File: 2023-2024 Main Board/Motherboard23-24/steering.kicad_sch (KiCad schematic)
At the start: 5 parts, among them J1 Conn_01x06_Pin, J18 Conn_01x02_Pin, J19 Conn_01x03_Pin, J7 Conn_01x03_Pin, U1 ARDUINO_PRO_MINI

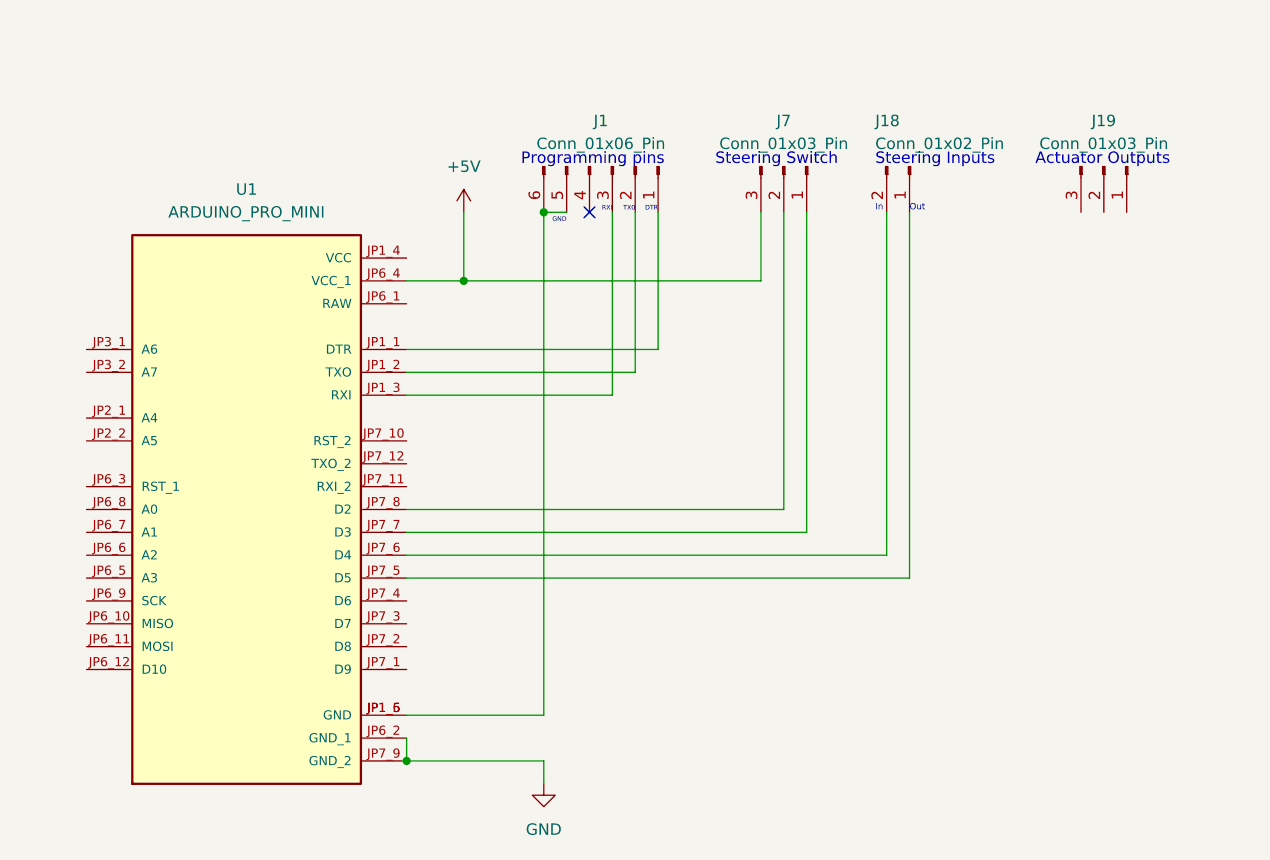
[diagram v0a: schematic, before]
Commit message: Added BOM
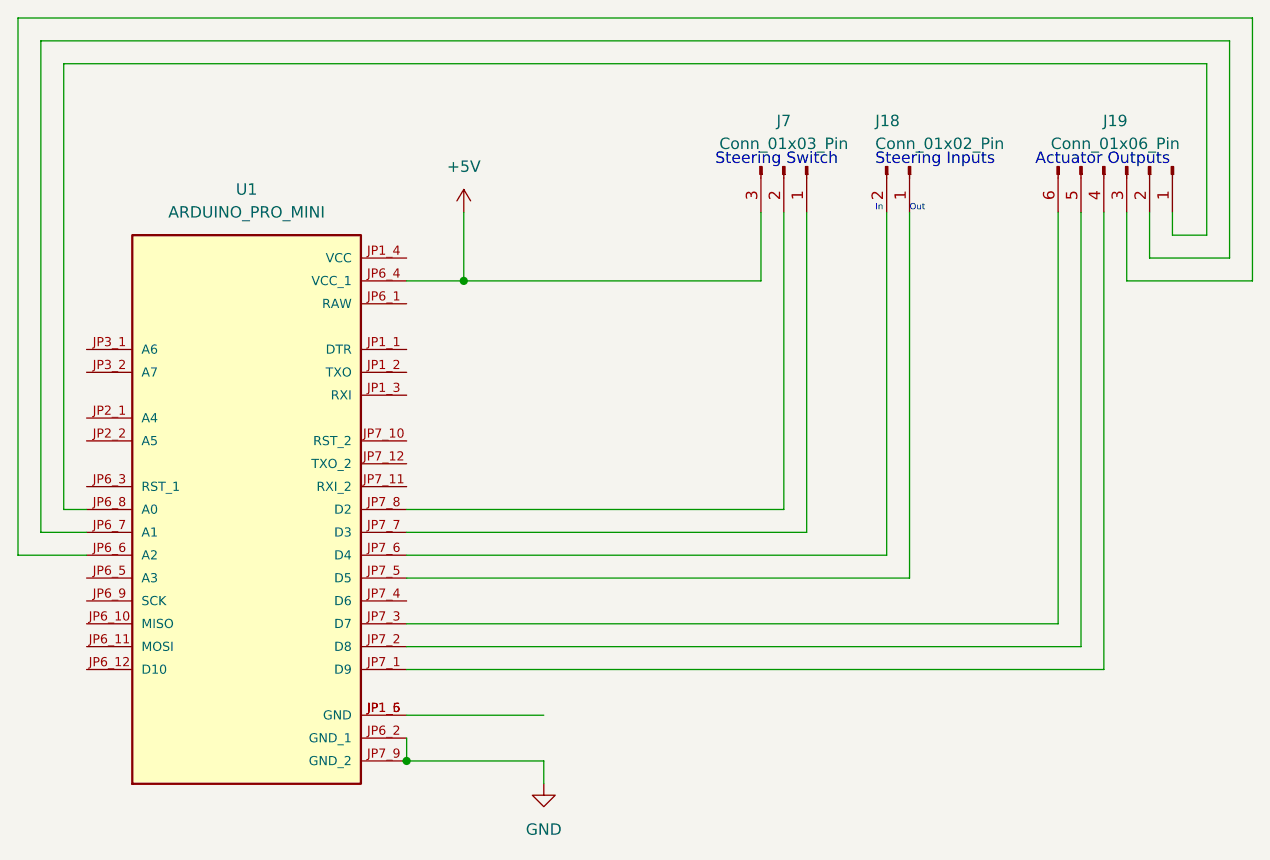
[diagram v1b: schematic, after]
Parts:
- removed J1: Conn_01x06_Pin, symbol Connector:Conn_01x06_Pin
- removed J19: Conn_01x03_Pin, symbol Connector:Conn_01x03_Pin
- added J19: Conn_01x06_Pin, symbol Connector:Conn_01x06_Pin
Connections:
- net at U1.JP6_6 (A2): now also J19.3 (Pin_3)
- net at U1.JP6_7 (A1): now also J19.2 (Pin_2)
- net at U1.JP6_8 (A0): now also J19.1 (Pin_1)
- net at U1.JP7_1 (D9): now also J19.4 (Pin_4)
- net at U1.JP7_2 (D8): now also J19.5 (Pin_5)
- net at U1.JP7_3 (D7): now also J19.6 (Pin_6)
- no-connect marks 1 -> 0
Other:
- note removed: "DTR"
- note removed: "GND"
- note removed: "Programming pins"
- note removed: "RXI"
- note removed: "TX0"
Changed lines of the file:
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@@
   (junction (at 116.84 86.36) (diameter 0) (color 0 0 0 0)
   )
-  (junction (at 125.73 78.74) (diameter 0) (color 0 0 0 0)
-  )
-  (no_connect (at 130.81 78.74))
+  (wire (pts (xy 69.85 59.69) (xy 69.85 114.3))
+    (stroke (width 0) (type default))
+  )
+  (wire (pts (xy 201.93 83.82) (xy 201.93 59.69))
+    (stroke (width 0) (type default))
+  )
   (wire (pts (xy 149.86 86.36) (xy 149.86 78.74))
     (stroke (width 0) (type default))
   )
-  (wire (pts (xy 125.73 78.74) (xy 128.27 78.74))
+  (wire (pts (xy 187.96 78.74) (xy 187.96 129.54))
     (stroke (width 0) (type default))
   )
@@
     (stroke (width 0) (type default))
   )
-  (wire (pts (xy 125.73 78.74) (xy 125.73 134.62))
+  (wire (pts (xy 182.88 78.74) (xy 182.88 124.46))
+    (stroke (width 0) (type default))
+  )
+  (wire (pts (xy 185.42 127) (xy 110.49 127))
     (stroke (width 0) (type default))
   )
@@
     (stroke (width 0) (type default))
   )
+  (wire (pts (xy 199.39 81.28) (xy 199.39 62.23))
+    (stroke (width 0) (type default))
+  )
+  (wire (pts (xy 72.39 111.76) (xy 74.93 111.76))
+    (stroke (width 0) (type default))
+  )
+  (wire (pts (xy 195.58 81.28) (xy 199.39 81.28))
+    (stroke (width 0) (type default))
+  )
   (wire (pts (xy 154.94 78.74) (xy 154.94 114.3))
     (stroke (width 0) (type default))
   )
-  (wire (pts (xy 138.43 78.74) (xy 138.43 93.98))
-    (stroke (width 0) (type default))
-  )
-  (wire (pts (xy 110.49 96.52) (xy 135.89 96.52))
+  (wire (pts (xy 187.96 129.54) (xy 110.49 129.54))
+    (stroke (width 0) (type default))
+  )
+  (wire (pts (xy 67.31 57.15) (xy 204.47 57.15))
+    (stroke (width 0) (type default))
+  )
+  (wire (pts (xy 72.39 62.23) (xy 199.39 62.23))
+    (stroke (width 0) (type default))
+  )
+  (wire (pts (xy 193.04 83.82) (xy 201.93 83.82))
+    (stroke (width 0) (type default))
+  )
+  (wire (pts (xy 67.31 57.15) (xy 67.31 116.84))
     (stroke (width 0) (type default))
   )
@@
     (stroke (width 0) (type default))
   )
+  (wire (pts (xy 69.85 59.69) (xy 201.93 59.69))
+    (stroke (width 0) (type default))
+  )
   (wire (pts (xy 110.49 86.36) (xy 116.84 86.36))
     (stroke (width 0) (type default))
   )
-  (wire (pts (xy 110.49 93.98) (xy 138.43 93.98))
-    (stroke (width 0) (type default))
-  )
-  (wire (pts (xy 133.35 78.74) (xy 133.35 99.06))
+  (wire (pts (xy 67.31 116.84) (xy 74.93 116.84))
+    (stroke (width 0) (type default))
+  )
+  (wire (pts (xy 190.5 86.36) (xy 204.47 86.36))
+    (stroke (width 0) (type default))
+  )
+  (wire (pts (xy 72.39 62.23) (xy 72.39 111.76))
+    (stroke (width 0) (type default))
+  )
+  (wire (pts (xy 204.47 86.36) (xy 204.47 57.15))
     (stroke (width 0) (type default))
   )
@@
     (stroke (width 0) (type default))
   )
+  (wire (pts (xy 193.04 78.74) (xy 193.04 83.82))
+    (stroke (width 0) (type default))
+  )
   (wire (pts (xy 125.73 139.7) (xy 125.73 142.24))
     (stroke (width 0) (type default))
   )
-  (wire (pts (xy 110.49 99.06) (xy 133.35 99.06))
+  (wire (pts (xy 190.5 78.74) (xy 190.5 86.36))
+    (stroke (width 0) (type default))
+  )
+  (wire (pts (xy 69.85 114.3) (xy 74.93 114.3))
     (stroke (width 0) (type default))
   )
@@
     (stroke (width 0) (type default))
   )
-  (wire (pts (xy 135.89 78.74) (xy 135.89 96.52))
-    (stroke (width 0) (type default))
-  )
   (wire (pts (xy 154.94 114.3) (xy 110.49 114.3))
     (stroke (width 0) (type default))
   )
+  (wire (pts (xy 185.42 78.74) (xy 185.42 127))
+    (stroke (width 0) (type default))
+  )
   (wire (pts (xy 152.4 111.76) (xy 152.4 78.74))
     (stroke (width 0) (type default))
   )
-  (text "RXI" (at 133.35 78.74 0)
-    (effects (font (size 0.508 0.508)) (justify right bottom))
+  (wire (pts (xy 195.58 78.74) (xy 195.58 81.28))
+    (stroke (width 0) (type default))
+  )
+  (wire (pts (xy 182.88 124.46) (xy 110.49 124.46))
+    (stroke (width 0) (type default))
   )
   (text "Steering Switch" (at 144.78 73.66 0)
     (effects (font (size 1.27 1.27)) (justify left bottom))
   )
-  (text "DTR" (at 138.43 78.74 0)
-    (effects (font (size 0.508 0.508)) (justify right bottom))
-  )
   (text "Out" (at 166.37 78.74 0)
     (effects (font (size 0.7 0.7)) (justify left bottom))
   )
-  (text "GND" (at 128.27 80.01 0)
-    (effects (font (size 0.508 0.508)) (justify right bottom))
-  )
-  (text "TX0" (at 135.89 78.74 0)
-    (effects (font (size 0.508 0.508)) (justify right bottom))
-  )
   (text "Actuator Outputs" (at 180.34 73.66 0)
     (effects (font (size 1.27 1.27)) (justify left bottom))
@@
     (effects (font (size 1.27 1.27)) (justify left bottom))
   )
-  (text "Programming pins " (at 123.19 73.66 0)
-    (effects (font (size 1.27 1.27)) (justify left bottom))
-  )
   (text "In" (at 162.56 78.74 0)
     (effects (font (size 0.7 0.7)) (justify left bottom))
@@
     )
   )
-  (symbol (lib_id "Connector:Conn_01x06_Pin") (at 133.35 73.66 270) (unit 1)
-    (in_bom yes) (on_board yes) (dnp no) (fields_autoplaced)
-    (property "Reference" "J1" (at 132.08 68.58 90)
-      (effects (font (size 1.27 1.27)))
-    )
-    (property "Value" "Conn_01x06_Pin" (at 132.08 71.12 90)
-      (effects (font (size 1.27 1.27)))
-    )
-    (property "Footprint" "" (at 133.35 73.66 0)
-      (effects (font (size 1.27 1.27)) hide)
-    )
-    (property "Datasheet" "~" (at 133.35 73.66 0)
+  (symbol (lib_id "power:+5V") (at 116.84 78.74 0) (unit 1)
+    (in_bom yes) (on_board yes) (dnp no) (fields_autoplaced)
+    (property "Reference" "#PWR02" (at 116.84 82.55 0)
+      (effects (font (size 1.27 1.27)) hide)
+    )
+    (property "Value" "+5V" (at 116.84 73.66 0)
+      (effects (font (size 1.27 1.27)))
+    )
+    (property "Footprint" "" (at 116.84 78.74 0)
+      (effects (font (size 1.27 1.27)) hide)
+    )
+    (property "Datasheet" "" (at 116.84 78.74 0)
+      (effects (font (size 1.27 1.27)) hide)
+    )
+    (pin "1")
+    (instances
+      (project "Motherboard23-24"
+        (path "/418d1727-08ff-41e8-954f-e6e13e4fb4ca/97542c42-a706-445d-a930-fc308481bbac"
+          (reference "#PWR02") (unit 1)
+        )
+      )
+    )
+  )
+  (symbol (lib_id "Connector:Conn_01x06_Pin") (at 190.5 73.66 270) (unit 1)
+    (in_bom yes) (on_board yes) (dnp no) (fields_autoplaced)
+    (property "Reference" "J19" (at 189.23 68.58 90)
+      (effects (font (size 1.27 1.27)))
+    )
+    (property "Value" "Conn_01x06_Pin" (at 189.23 71.12 90)
+      (effects (font (size 1.27 1.27)))
+    )
+    (property "Footprint" "" (at 190.5 73.66 0)
+      (effects (font (size 1.27 1.27)) hide)
+    )
+    (property "Datasheet" "~" (at 190.5 73.66 0)
       (effects (font (size 1.27 1.27)) hide)
     )
@@
       (project "Motherboard23-24"
         (path "/418d1727-08ff-41e8-954f-e6e13e4fb4ca/97542c42-a706-445d-a930-fc308481bbac"
-          (reference "J1") (unit 1)
+          (reference "J19") (unit 1)
         )
         (path "/418d1727-08ff-41e8-954f-e6e13e4fb4ca/d15f88a3-eb3a-4abd-b913-7ade9bdcdd4a"
           (reference "J8") (unit 1)
-        )
-      )
-    )
-  )
-  (symbol (lib_id "power:+5V") (at 116.84 78.74 0) (unit 1)
-    (in_bom yes) (on_board yes) (dnp no) (fields_autoplaced)
-    (property "Reference" "#PWR02" (at 116.84 82.55 0)
-      (effects (font (size 1.27 1.27)) hide)
-    )
-    (property "Value" "+5V" (at 116.84 73.66 0)
-      (effects (font (size 1.27 1.27)))
-    )
-    (property "Footprint" "" (at 116.84 78.74 0)
-      (effects (font (size 1.27 1.27)) hide)
-    )
-    (property "Datasheet" "" (at 116.84 78.74 0)
-      (effects (font (size 1.27 1.27)) hide)
-    )
-    (pin "1")
-    (instances
-      (project "Motherboard23-24"
-        (path "/418d1727-08ff-41e8-954f-e6e13e4fb4ca/97542c42-a706-445d-a930-fc308481bbac"
-          (reference "#PWR02") (unit 1)
         )
       )
@@
         )
       )
-    )
-  )
-  (symbol (lib_id "Connector:Conn_01x03_Pin") (at 187.96 73.66 270) (unit 1)
-    (in_bom yes) (on_board yes) (dnp no) (fields_autoplaced)
-    (property "Reference" "J19" (at 187.96 68.58 90)
-      (effects (font (size 1.27 1.27)))
-    )
-    (property "Value" "Conn_01x03_Pin" (at 187.96 71.12 90)
-      (effects (font (size 1.27 1.27)))
-    )
-    (property "Footprint" "" (at 187.96 73.66 0)
-      (effects (font (size 1.27 1.27)) hide)
-    )
-    (property "Datasheet" "~" (at 187.96 73.66 0)
-      (effects (font (size 1.27 1.27)) hide)
-    )
-    (pin "1")
-    (pin "2")
-    (pin "3")
-    (instances
-      (project "Motherboard23-24"
-        (path "/418d1727-08ff-41e8-954f-e6e13e4fb4ca/97542c42-a706-445d-a930-fc308481bbac"
-          (reference "J19") (unit 1)
-        )
-      )
